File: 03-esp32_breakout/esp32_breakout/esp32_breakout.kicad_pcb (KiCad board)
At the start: 4 copper layers, 39.2 x 22.8 mm, 44 parts, among them J1 USB4110-GF-A, J2 Conn_01x06, SW1 SW_Push, SW2 SW_Push, SW3 SW_Push, U1 ESP32-S3, U3 AP2112H, Y1 ECS-400-10-37B2-CKY-TR, Y2 ECS-.327-12.5-34B-TR

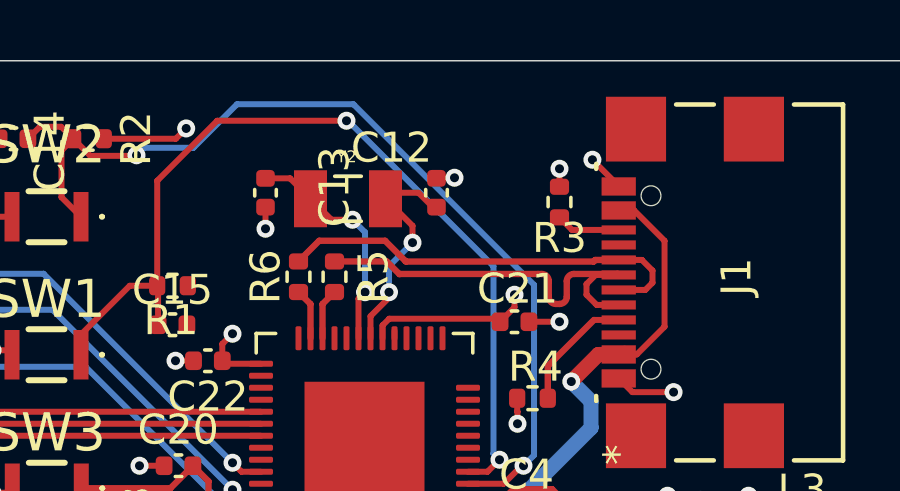
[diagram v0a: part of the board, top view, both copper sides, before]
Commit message: ground zone
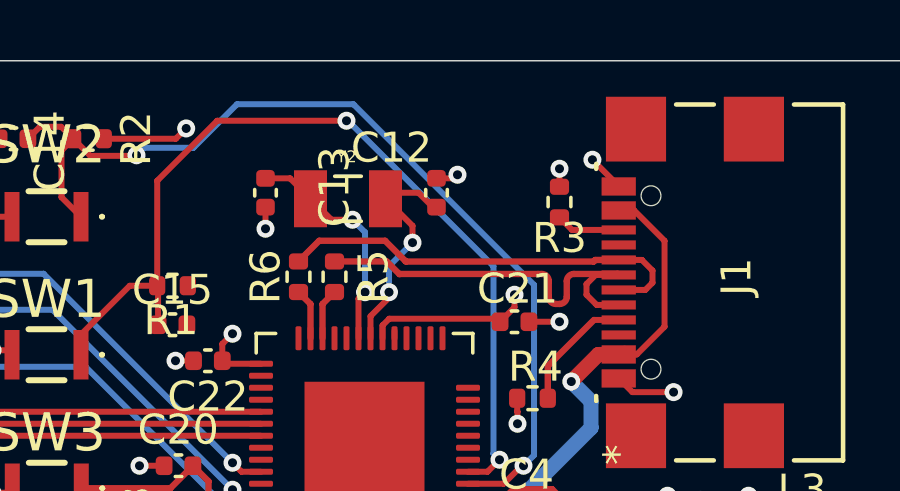
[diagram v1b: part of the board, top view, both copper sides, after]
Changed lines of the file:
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@@
+	)
+	(segment
+		(start 168.18 51.92)
+		(end 167.6 51.92)
+		(width 0.2)
+		(layer "F.Cu")
+		(net 1)
 	)
 	(segment
@@
 	)
 	(segment
-		(start 168.18 51.92)
-		(end 168.2 51.9)
-		(width 0.2)
-		(layer "F.Cu")
-		(net 1)
-	)
-	(segment
 		(start 177.985 63.115)
 		(end 177.985 62.515)
@@
 	)
 	(segment
+		(start 168.3 51.8)
+		(end 168.18 51.92)
+		(width 0.2)
+		(layer "F.Cu")
+		(net 1)
+	)
+	(segment
 		(start 177.985 62.515)
 		(end 178 62.5)
@@
 	)
 	(segment
-		(start 167.6 51.92)
-		(end 168.18 51.92)
-		(width 0.2)
-		(layer "F.Cu")
-		(net 1)
-	)
-	(segment
 		(start 170.29 59.69)
 		(end 170.29 59.25)
@@
 	)
 	(via
-		(at 168.2 51.9)
+		(at 168.3 51.8)
 		(size 0.6)
 		(drill 0.3)
@@
 		(polygon
 			(pts
-				(xy 156.6 22.6) (xy 157 36) (xy 178.8 35.9) (xy 177.1 21.7)
-			)
-		)
-	)
-	(zone
-		(net 0)
-		(net_name "")
-		(layer "In1.Cu")
-		(hatch edge 0.5)
-		(connect_pads
-			(clearance 0)
-		)
-		(min_thickness 0.25)
-		(filled_areas_thickness no)
-		(keepout
-			(tracks allowed)
-			(vias allowed)
-			(pads allowed)
-			(copperpour not_allowed)
-			(footprints allowed)
-		)
-		(placement
-			(enabled no)
-			(sheetname "/")
-		)
-		(fill
-			(thermal_gap 0.5)
-			(thermal_bridge_width 0.5)
-		)
-		(polygon
-			(pts
-				(xy 160.9 50.8) (xy 168.9 50.8) (xy 168.9 57.9) (xy 160.9 57.8)
+				(xy 161.3 51.3) (xy 168.6 51.3) (xy 168.6 57.6) (xy 161.3 57.5)
 			)
 		)
@@
 		(polygon
 			(pts
-				(xy 140.75 44) (xy 192 43.5) (xy 192 78) (xy 139.25 77)
+				(xy 192 78) (xy 139.25 77) (xy 140.75 44) (xy 192 43.5)
 			)
 		)
+		(polygon
+			(pts
+				(xy 162.5 63.6) (xy 162.5 70) (xy 167.5 69.9) (xy 167.5 63.5)
+			)
+		)
+		(polygon
+			(pts
+				(xy 160.9 57.9) (xy 168.9 57.9) (xy 168.9 50.7) (xy 160.9 50.7)
+			)
+		)
+	)
+	(zone
+		(net 1)
+		(net_name "GND")
+		(layer "In1.Cu")
+		(hatch edge 0.5)
+		(priority 3)
+		(connect_pads yes
+			(clearance 0)
+		)
+		(min_thickness 0.25)
+		(filled_areas_thickness no)
+		(fill yes
+			(thermal_gap 0.5)
+			(thermal_bridge_width 0.5)
+		)
+		(polygon
+			(pts
+				(xy 167.3 63.8) (xy 167.3 69.5) (xy 162.8 69.5) (xy 162.8 63.8)
+			)
+		)
